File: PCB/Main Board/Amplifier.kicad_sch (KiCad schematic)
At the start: 48 parts, among them U10 OPA2197xD, U11 DG201, U7 DG201, U8 INA828D, U9 OPA2197xD

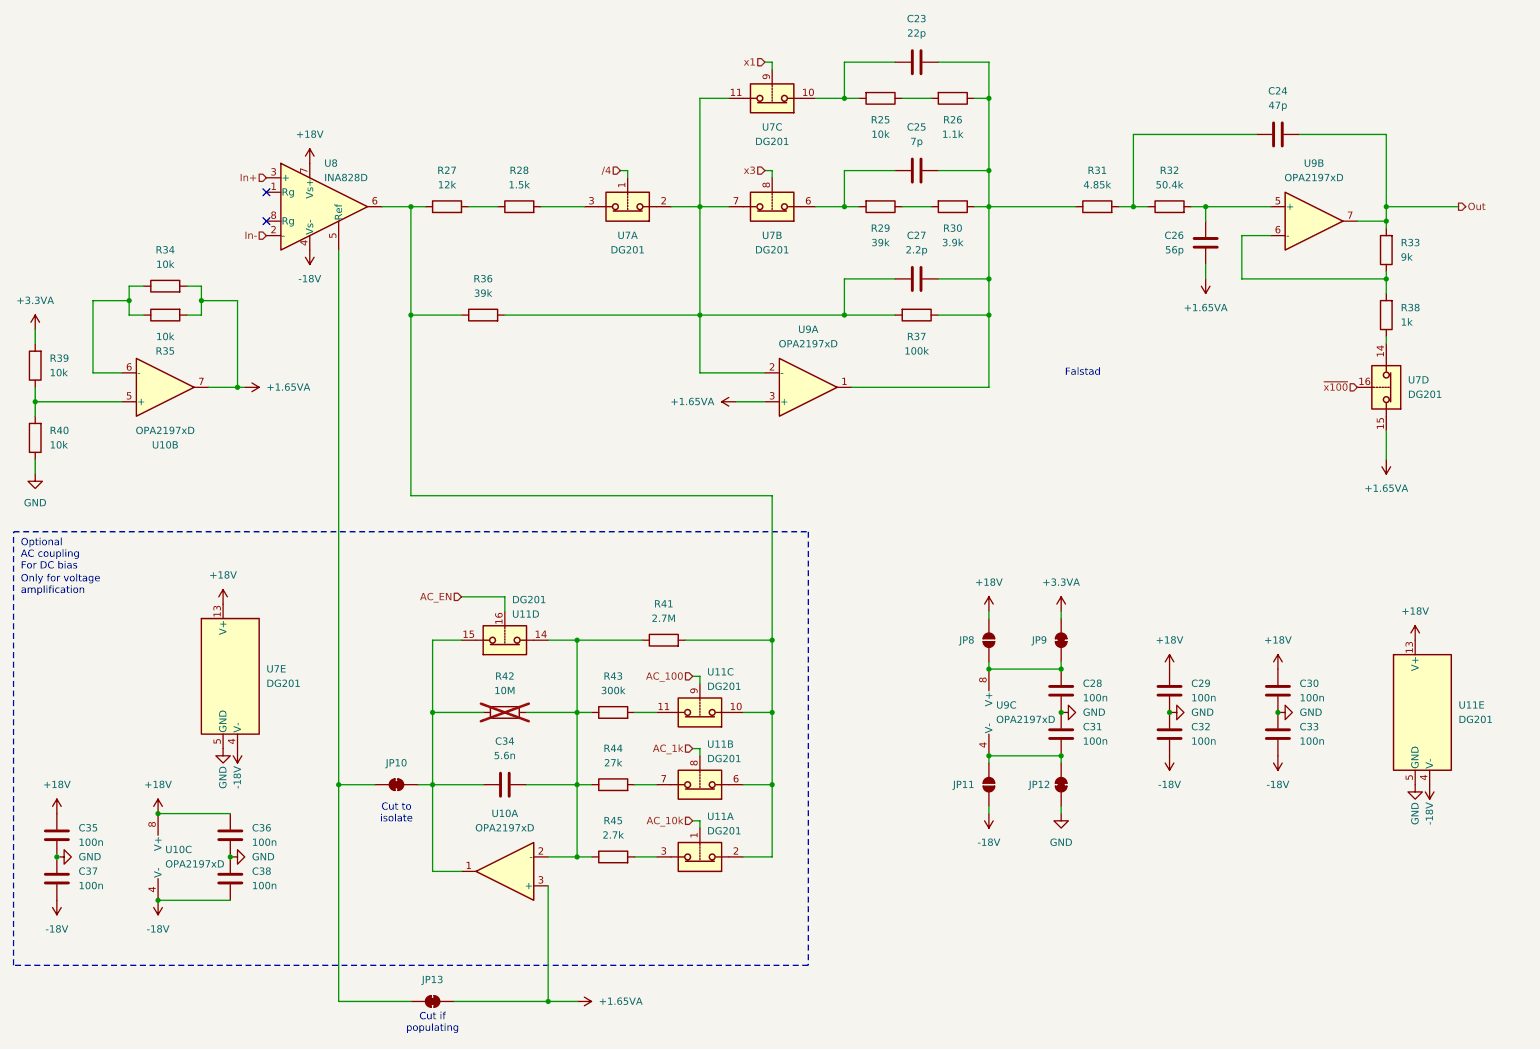
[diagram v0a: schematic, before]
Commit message: minor
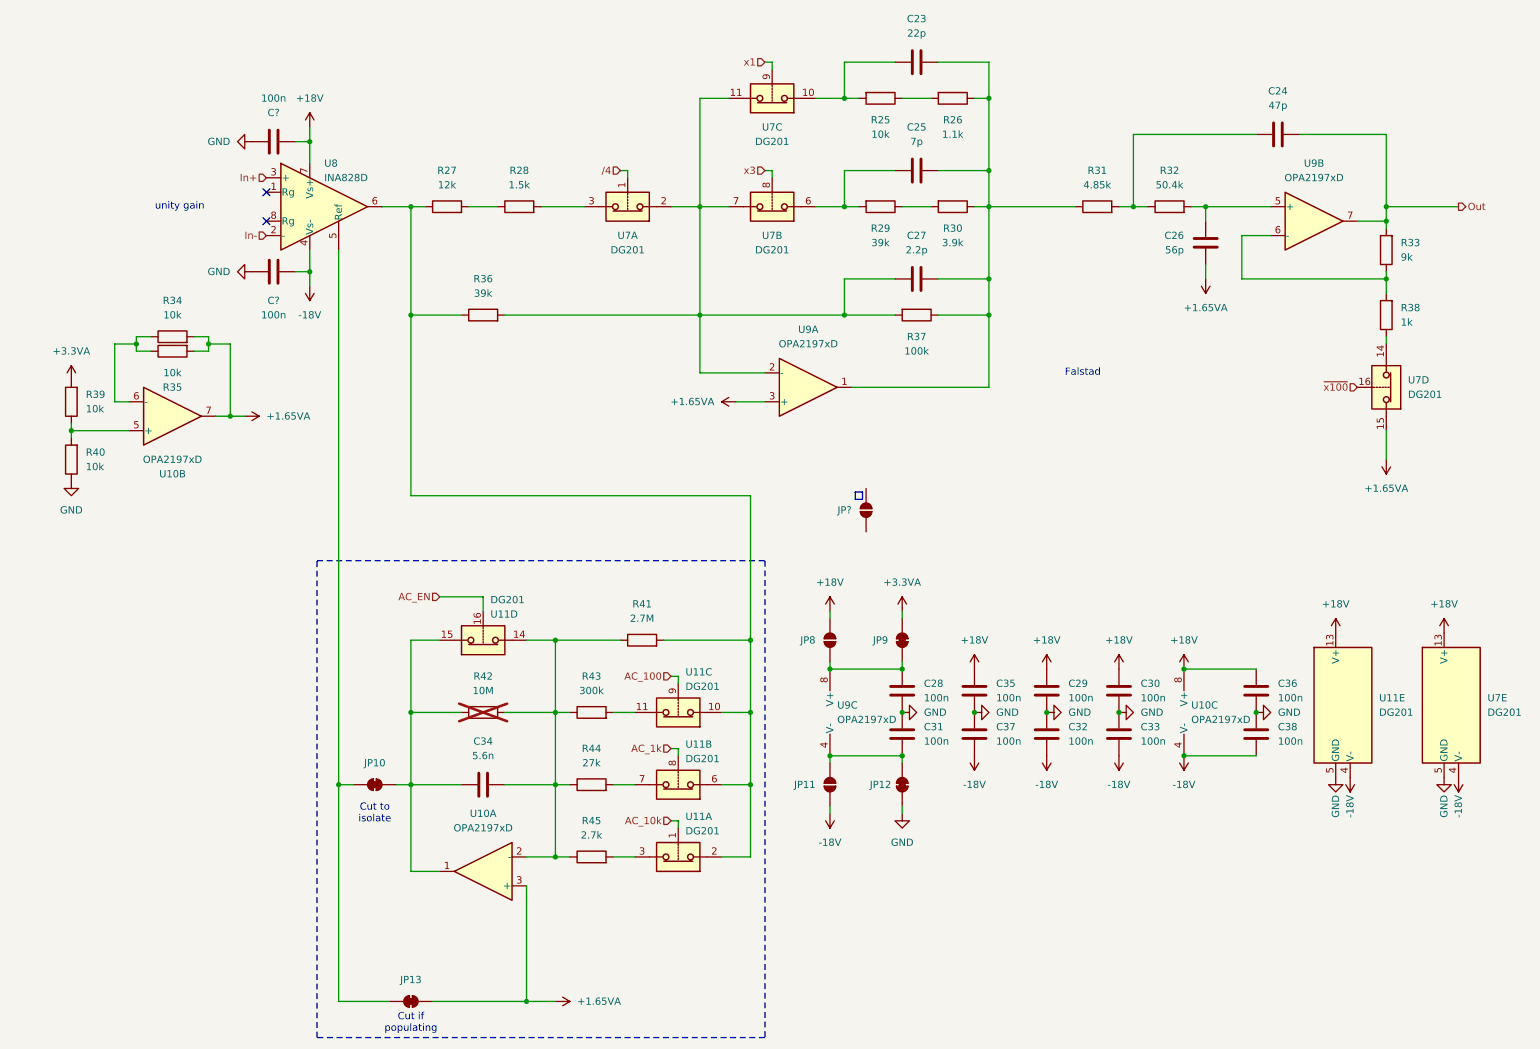
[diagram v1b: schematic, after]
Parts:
- added C? (x2): 100n, symbol Device:C
- added JP?: SolderJumper_2_Open, Jumper:SolderJumper-2_P1.3mm_Open_RoundedPad1.0x1.5mm, symbol Jumper:SolderJumper_2_Open
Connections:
- net +18V: now also C?.2
- net -18V: now also C?.2
- net GND: now also C?.1, C?.1
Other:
- note added: "unity gain"
- note removed: "Only for voltage amplification"
- note removed: "Optional AC coupling For DC bias"
- moved on the sheet: C28, C29, C30, C31, C32, C33, C34, C35, C36, C37, C38, JP10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
